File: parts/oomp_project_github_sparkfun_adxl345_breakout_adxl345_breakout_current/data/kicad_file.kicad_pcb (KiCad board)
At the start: 2 copper layers, 20.3 x 15.2 mm, 11 parts, among them U2 ADXL345PATRICK

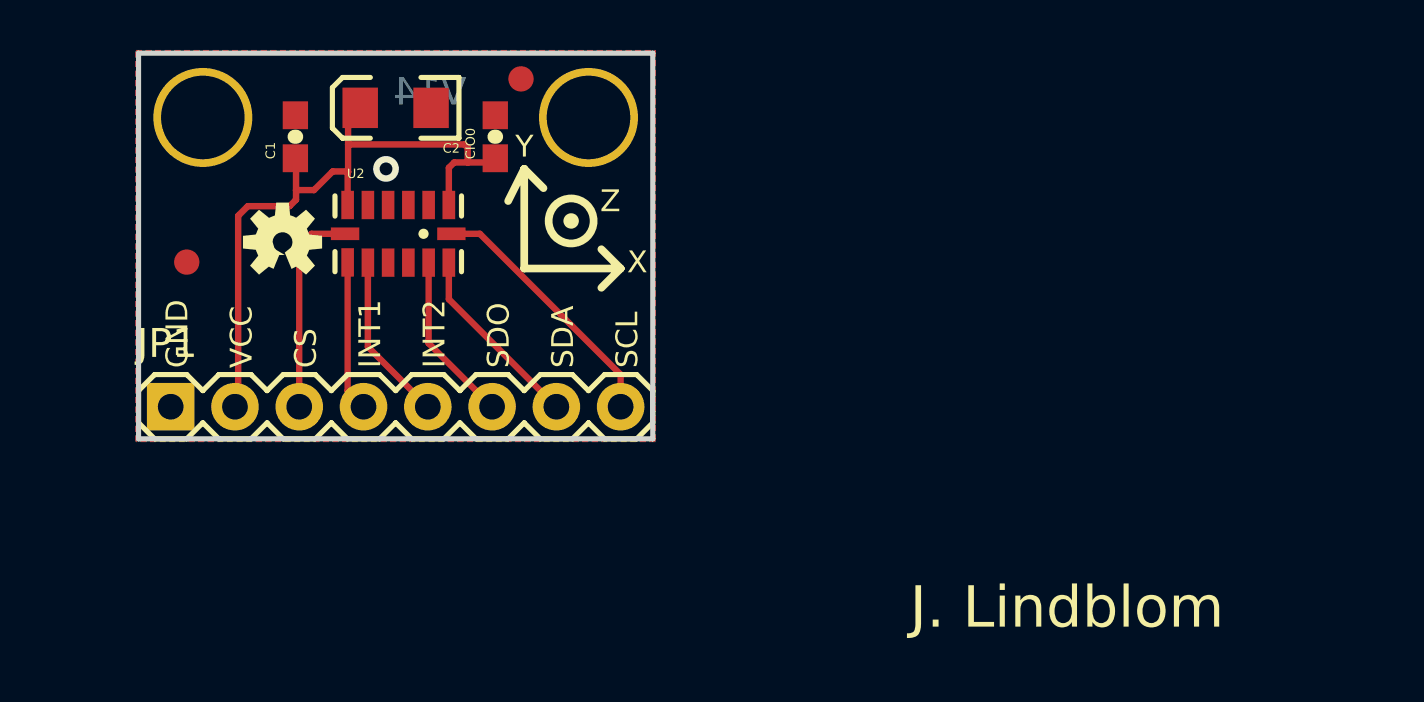
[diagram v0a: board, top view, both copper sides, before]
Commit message: working
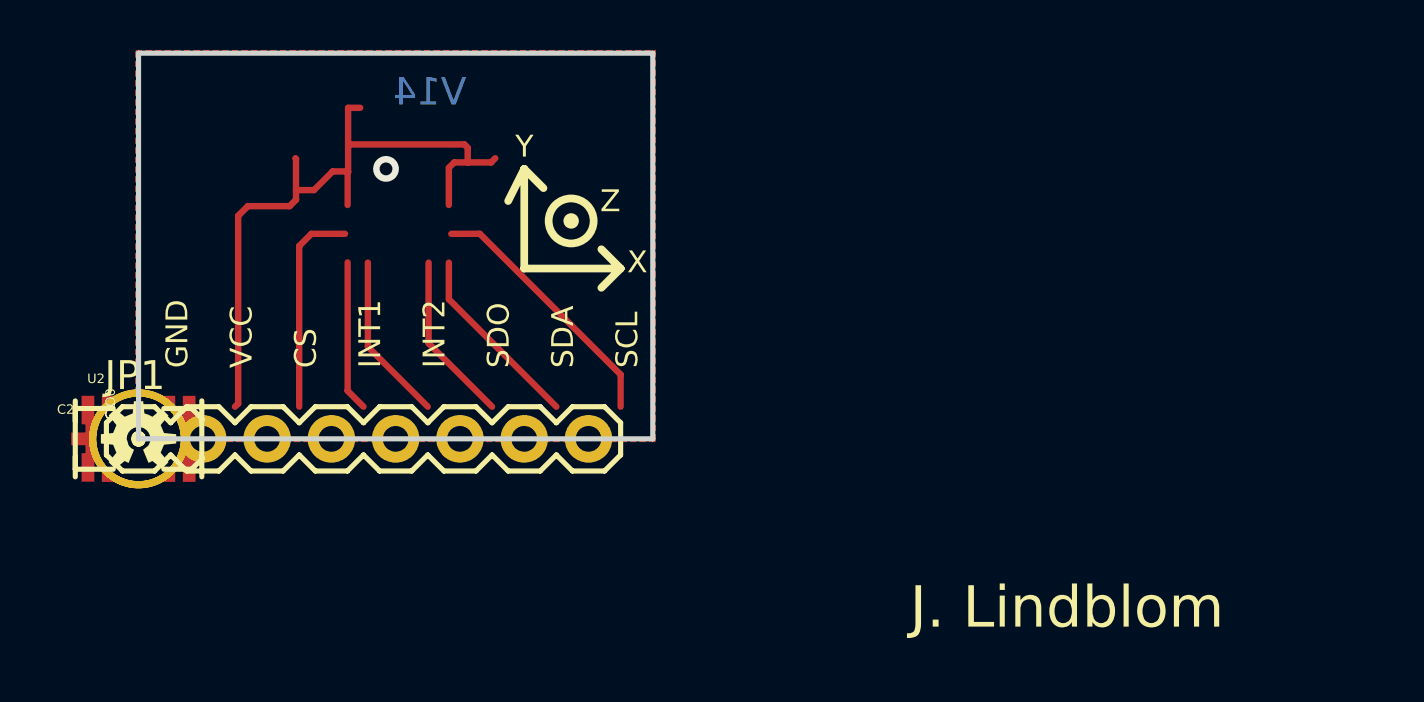
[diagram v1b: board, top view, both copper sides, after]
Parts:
- C1, CIO0: footprint 0603-CAP -> ADXL345_Breakout-import-fps:0603-CAP
- C2: footprint EIA3216 -> ADXL345_Breakout-import-fps:EIA3216
- JP1: footprint 1X08 -> ADXL345_Breakout-import-fps:1X08
- JP2, JP3: footprint STAND-OFF -> ADXL345_Breakout-import-fps:STAND-OFF
- JP4, JP5: footprint FIDUCIAL-1X2 -> ADXL345_Breakout-import-fps:FIDUCIAL-1X2
- U$2: footprint SFE-NEW-WEBLOGO -> ADXL345_Breakout-import-fps:SFE-NEW-WEBLOGO
- U$3: footprint OSHW-LOGO-S -> ADXL345_Breakout-import-fps:OSHW-LOGO-S
- U2: footprint LGA14_1_1_PATRICK -> ADXL345_Breakout-import-fps:LGA14_1_1_PATRICK
- moved JP3 21.8 mm to (0.00, 0.00)
- moved U$2 21.2 mm to (0.00, 0.00), turned to 0 degrees
- moved JP5 20.8 mm to (0.00, 0.00)
- moved CIO0 18.5 mm to (0.00, 0.00), turned to 0 degrees
- moved C2 16.6 mm to (0.00, 0.00), turned to 0 degrees
- moved C1 13.5 mm to (0.00, 0.00), turned to 0 degrees
- moved U2 13.1 mm to (0.00, 0.00)
- moved JP2 13.0 mm to (0.00, 0.00)
- moved U$3 9.63 mm to (0.00, 0.00)
- moved JP4 7.24 mm to (0.00, 0.00)
- moved JP1 1.80 mm to (0.00, 0.00)
